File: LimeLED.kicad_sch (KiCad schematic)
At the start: 20 parts, among them CN1 HB9500-3, CN2 HB9500-3, U1 ESP32-DEVKITC-32D, U2 TPSM863257RDXR, U3 220k, U4 SN74AHCT125N

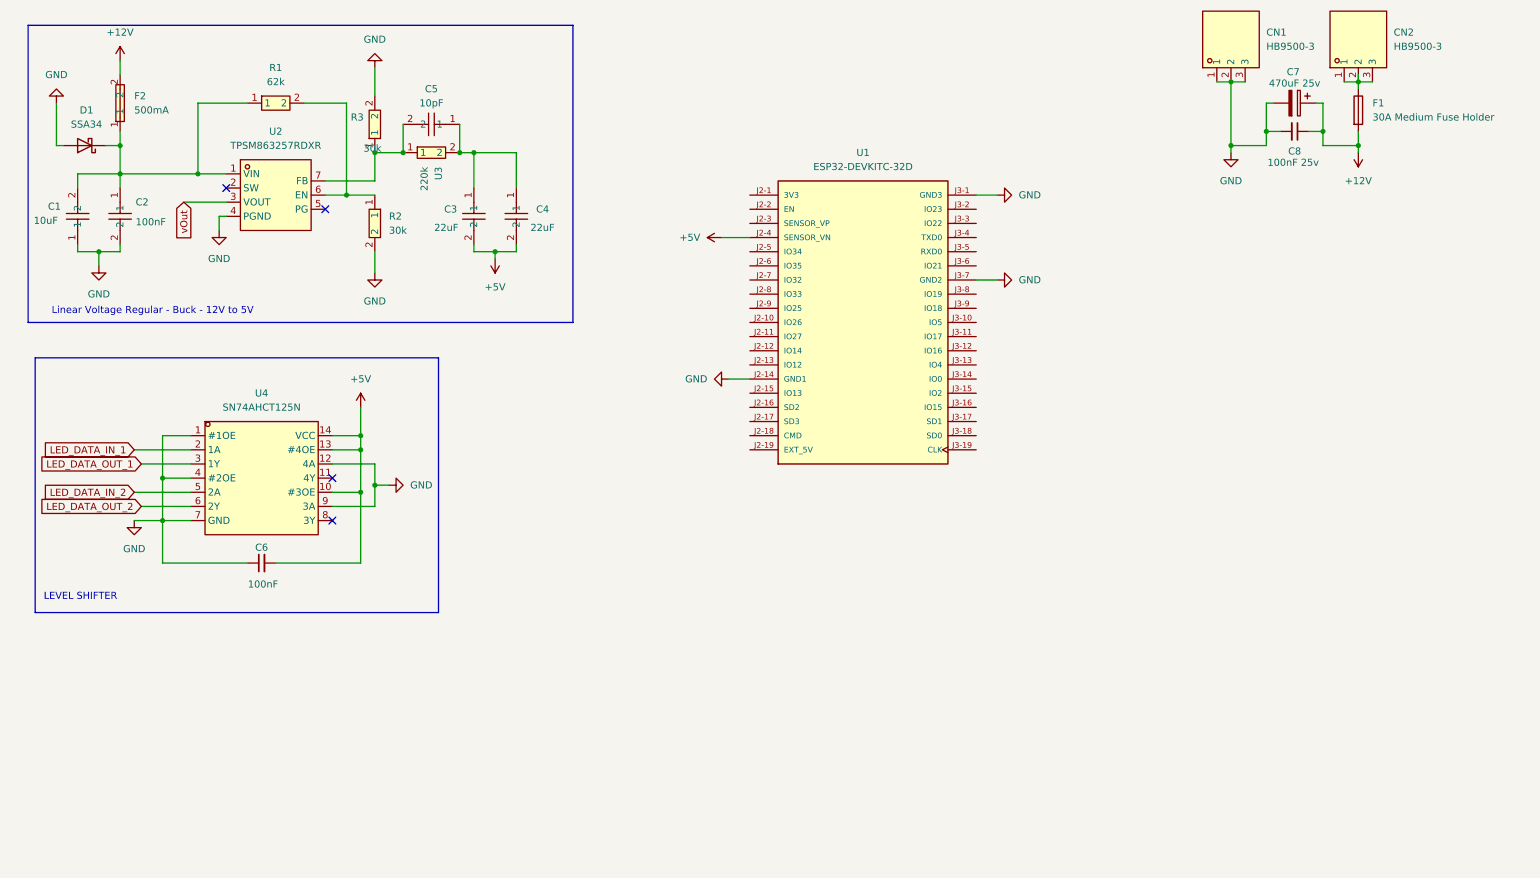
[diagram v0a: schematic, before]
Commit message: plot schematic
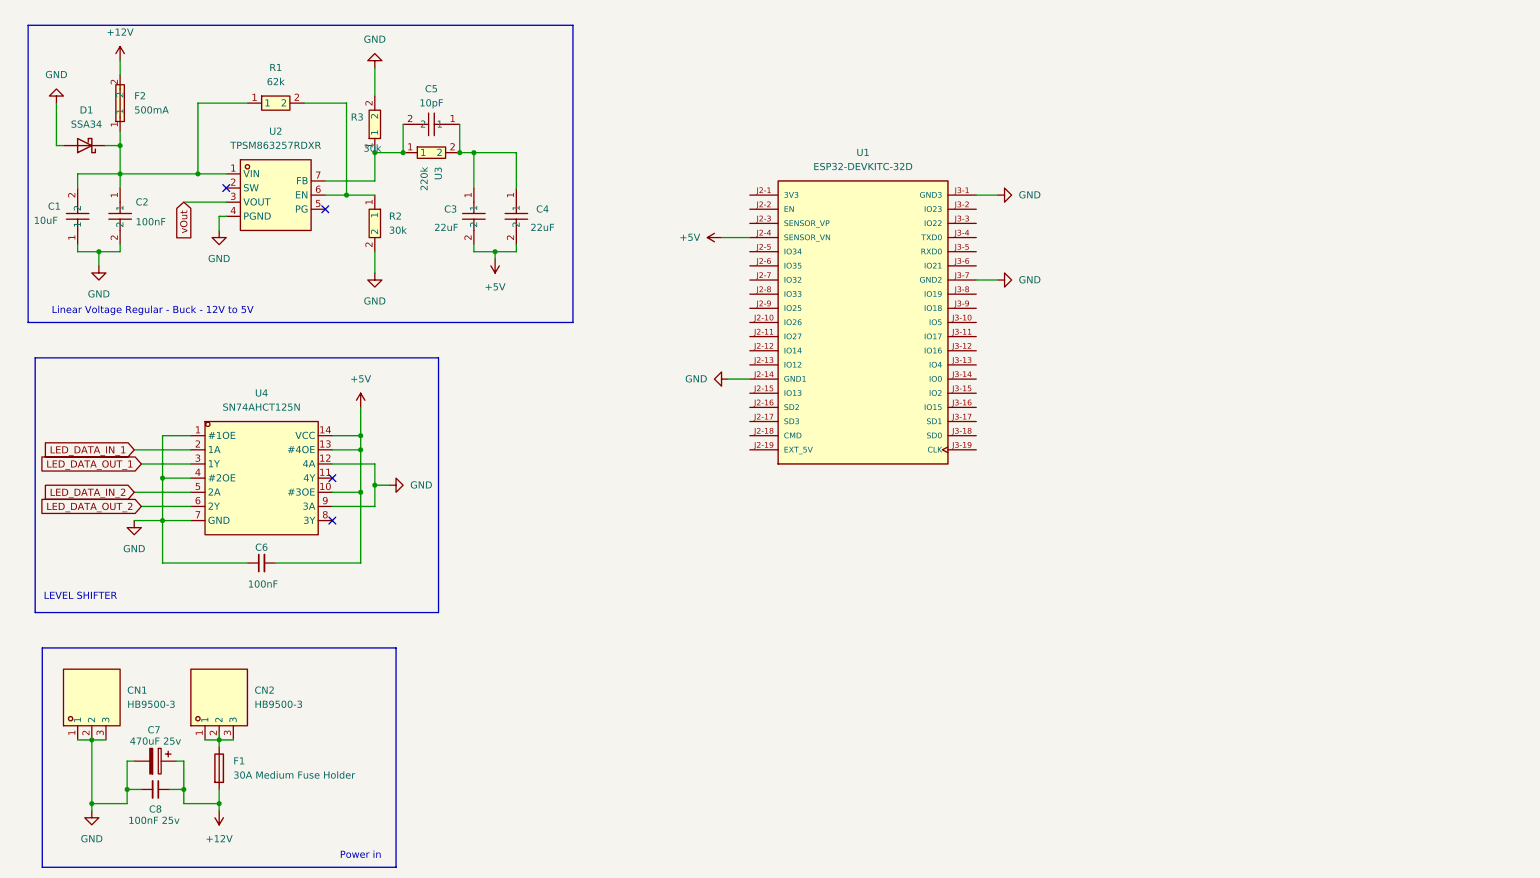
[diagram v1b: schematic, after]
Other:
- note added: "Power in"
- moved on the sheet: C7, C8, CN1, CN2, F1
